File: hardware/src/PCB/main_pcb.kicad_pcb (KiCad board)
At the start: 2 copper layers, 80 x 80 mm, 46 parts, among them J1 Batt, J2 Hall_sensor, J3 Pressure_sensor, J4 Pressure_pins, J5 converter_pins, Q2 BS170, Q4 IRF9530, Q5 IRF9530, Q6 IRF9530, SW1 Button, U2 XIAO-nRF52840-Plus-SMD

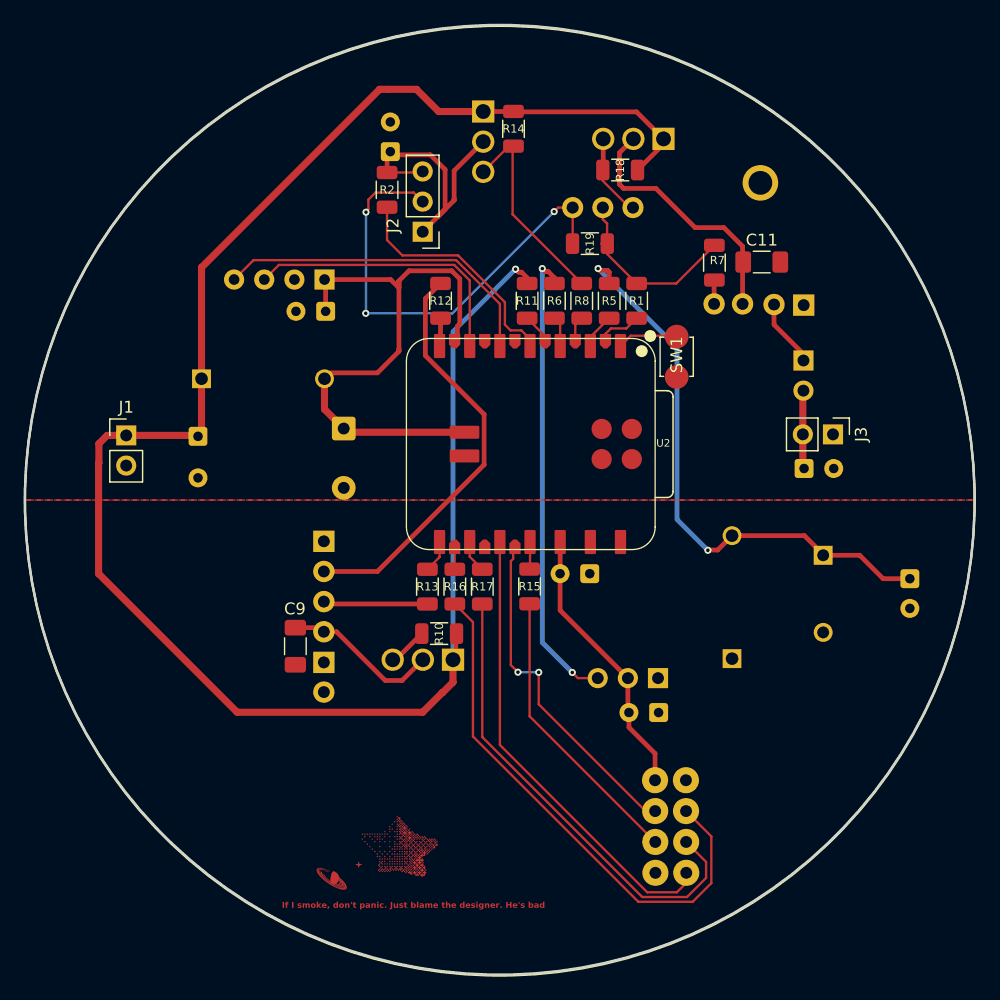
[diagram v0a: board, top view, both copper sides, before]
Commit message: feature: PCB ready to manufacture and firmeware start
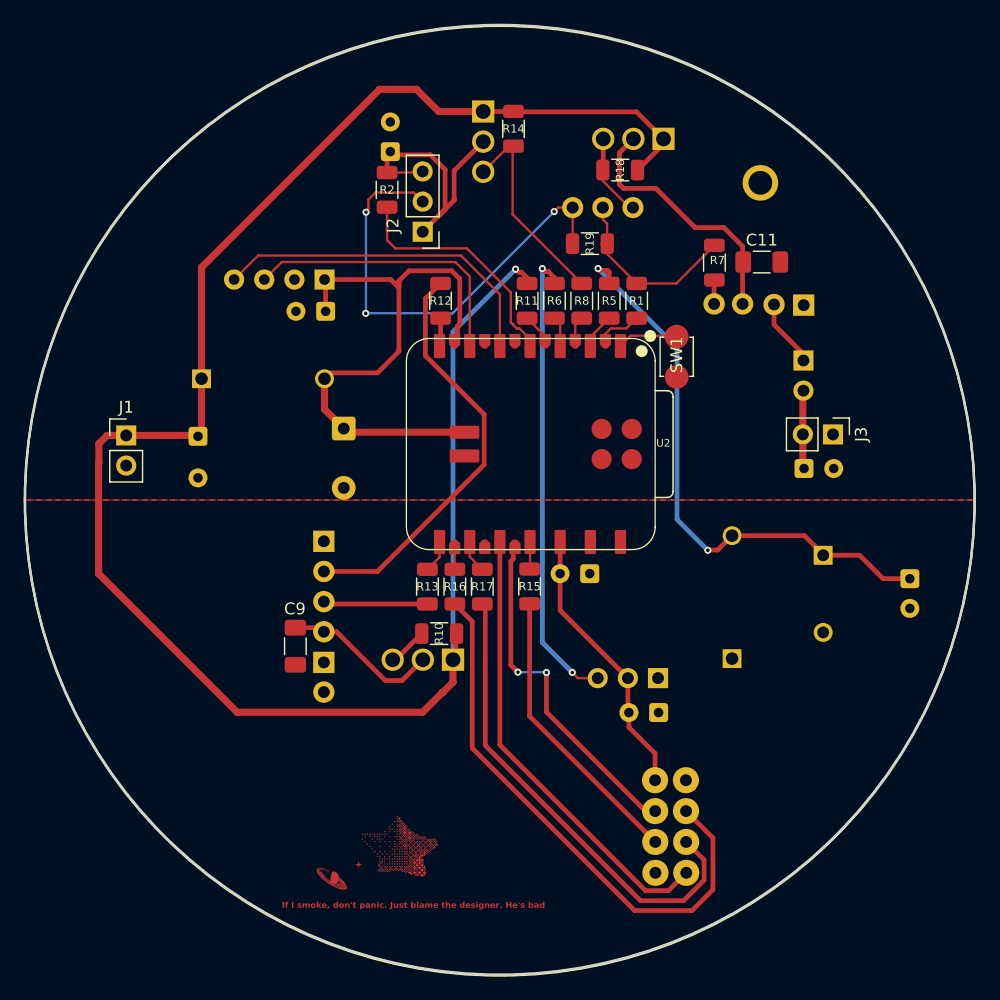
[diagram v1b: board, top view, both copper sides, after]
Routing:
- net /RF_GDO0: track 45.2 -> 47.0 mm
- net /SDA1: track 28.1 -> 28.9 mm
